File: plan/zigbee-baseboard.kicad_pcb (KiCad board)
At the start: 4 copper layers, 11.8 x 17.8 mm, 55 parts, among them J1 Debug_SWD_Pogo_2x3, J2 EFR32MG24_Core_Expansion_2x6, SW1 EVPBB2A9B000, U1 EFR32MG24B020F1536IM48-B, Y1 XTL501250-S315-038

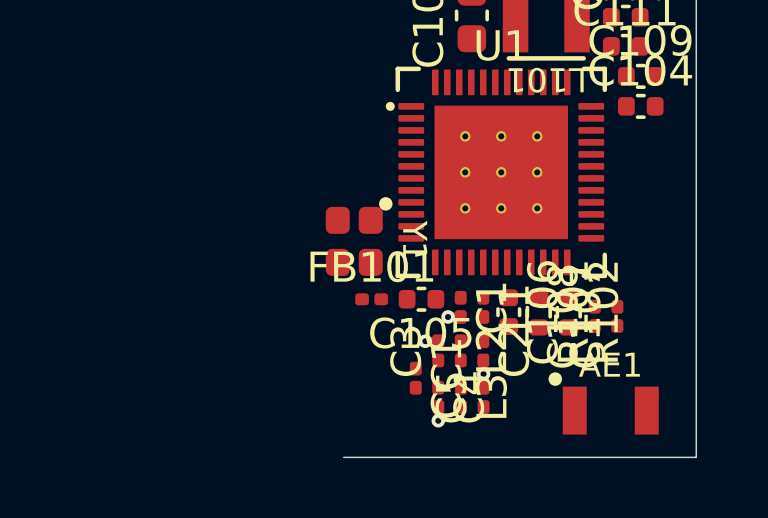
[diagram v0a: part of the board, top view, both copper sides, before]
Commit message: Route MG24 Matching network
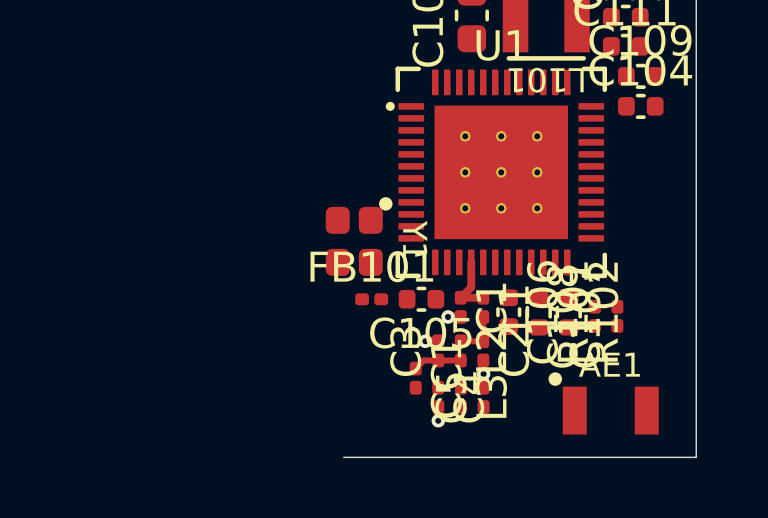
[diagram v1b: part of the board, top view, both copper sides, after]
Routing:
- net RF2G4_IO: track 0.00 -> 2.07 mm
- net Net-(C3-Pad1): track 0.00 -> 1.61 mm
- net Net-(C2-Pad1): track 0.00 -> 1.56 mm
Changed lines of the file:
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@@
 		(net "GND")
+	)
+	(segment
+		(start 142 97.33)
+		(end 141.65 97.68)
+		(width 0.2631)
+		(layer "F.Cu")
+		(net "RF2G4_IO")
+	)
+	(segment
+		(start 142 96.5)
+		(end 142 97.33)
+		(width 0.2631)
+		(layer "F.Cu")
+		(net "RF2G4_IO")
+	)
+	(segment
+		(start 141.65 97.68)
+		(end 142.4 97.68)
+		(width 0.2631)
+		(layer "F.Cu")
+		(net "RF2G4_IO")
+	)
+	(segment
+		(start 140.9 99.77)
+		(end 140.42 99.77)
+		(width 0.2)
+		(layer "F.Cu")
+		(net "Net-(C3-Pad1)")
+	)
+	(segment
+		(start 140.42 99.77)
+		(end 140.15 100.04)
+		(width 0.2)
+		(layer "F.Cu")
+		(net "Net-(C3-Pad1)")
+	)
+	(segment
+		(start 141.65 99.77)
+		(end 140.9 99.77)
+		(width 0.2)
+		(layer "F.Cu")
+		(net "Net-(C3-Pad1)")
+	)
+	(segment
+		(start 142.4 98.32)
+		(end 142.4 99.13)
+		(width 0.2)
+		(layer "F.Cu")
+		(net "Net-(C2-Pad1)")
+	)
+	(segment
+		(start 142.4 99.13)
+		(end 141.65 99.13)
+		(width 0.2)
+		(layer "F.Cu")
+		(net "Net-(C2-Pad1)")
 	)
 	(zone
